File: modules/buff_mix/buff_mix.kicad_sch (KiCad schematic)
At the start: 2 parts

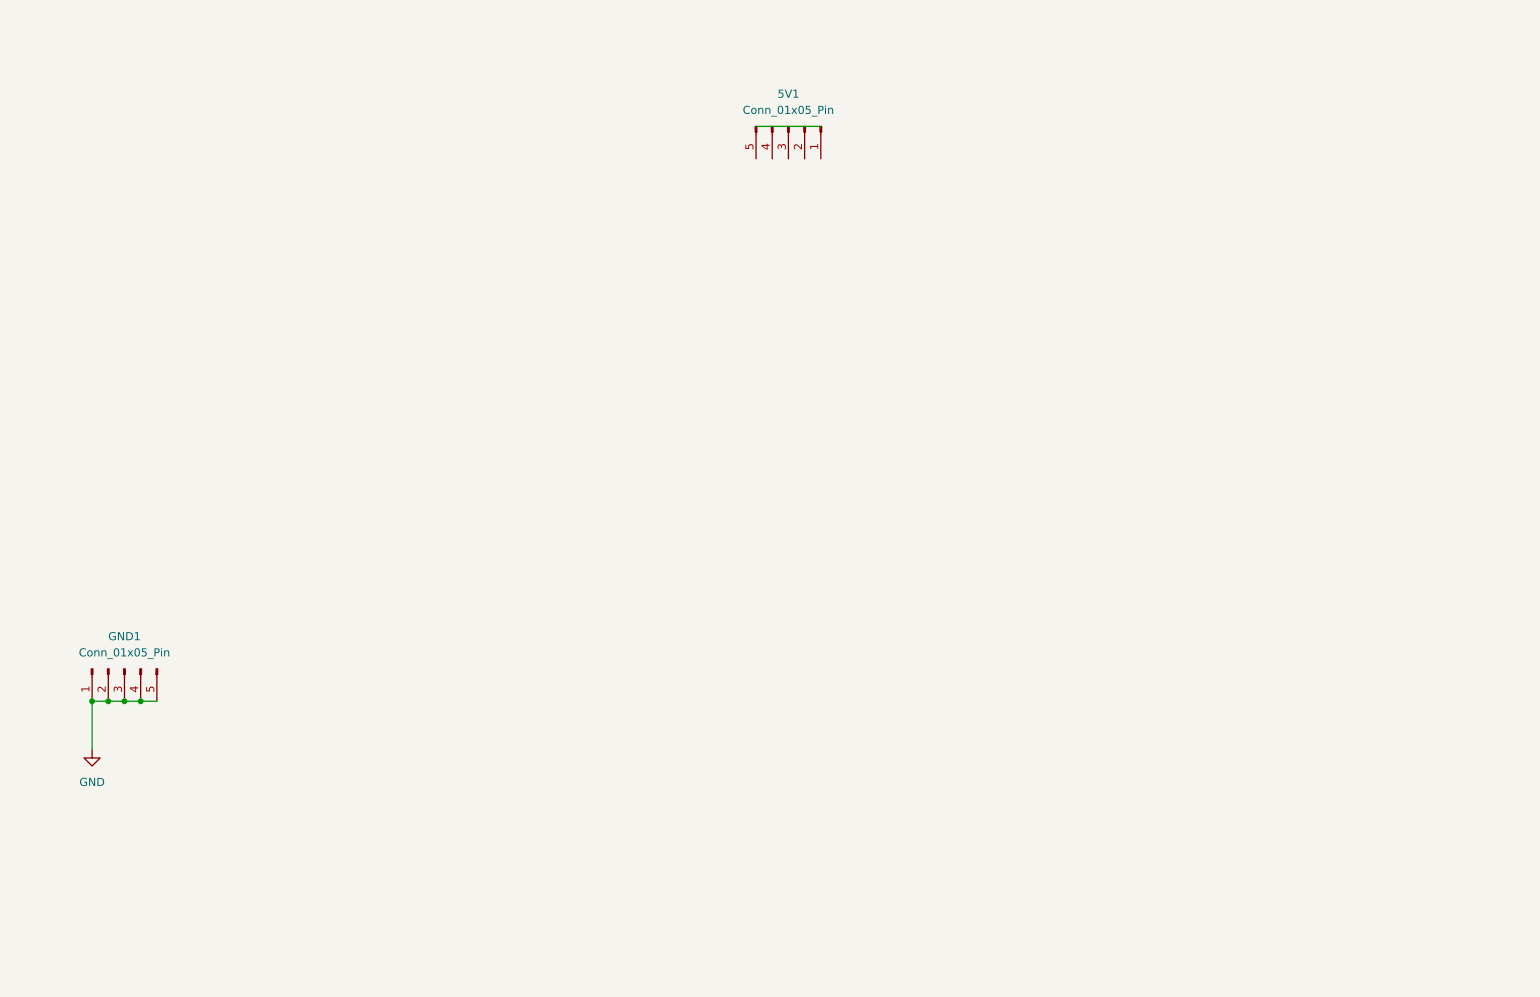
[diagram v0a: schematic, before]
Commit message: Add the final buff_mix
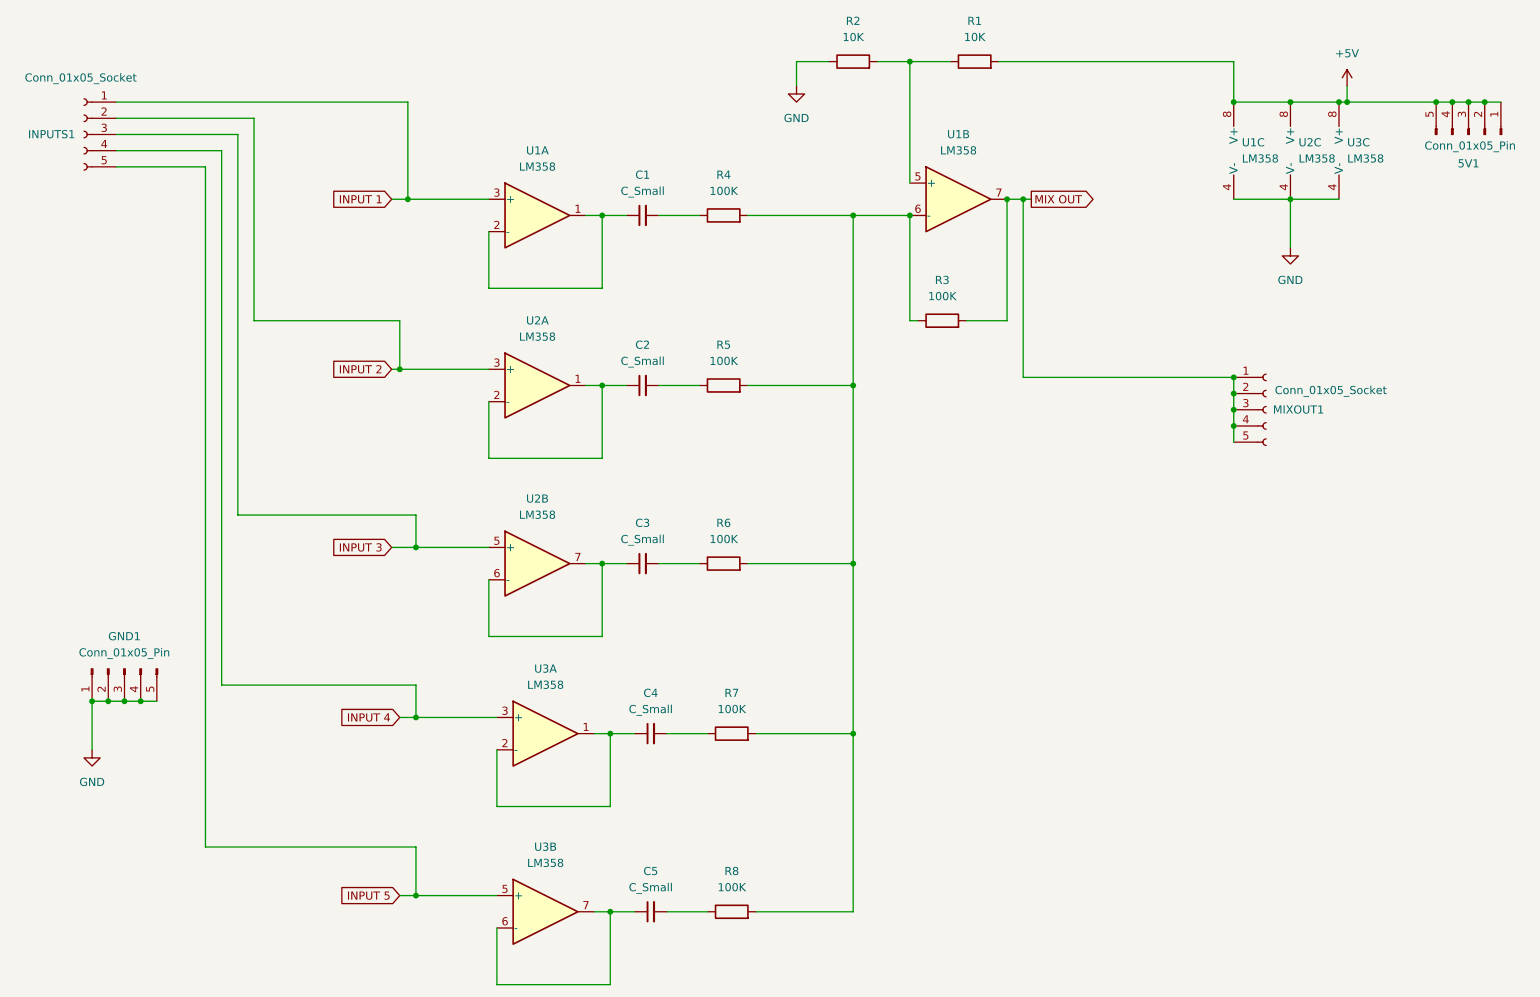
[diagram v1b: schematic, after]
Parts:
- added C1, C2, C3, C4, C5: C_Small, Capacitor_THT:C_Disc_D4.3mm_W1.9mm_P5.00mm, symbol Device:C_Small
- added INPUTS1, MIXOUT1: Conn_01x05_Socket, Connector_PinSocket_2.54mm:PinSocket_1x05_P2.54mm_Vertical, symbol Connector:Conn_01x05_Socket
- added R1, R2: 10K, Resistor_THT:R_Axial_DIN0207_L6.3mm_D2.5mm_P10.16mm_Horizontal, symbol Device:R
- added R3, R4, R5, R6, R7, R8: 100K, Resistor_THT:R_Axial_DIN0207_L6.3mm_D2.5mm_P10.16mm_Horizontal, symbol Device:R
- added U1, U2, U3: LM358, Library:LM358_THT, symbol Amplifier_Operational:LM358
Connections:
- net GND: now also R2.1, U1.4 (V-), U2.4 (V-), U3.4 (V-)
- net +5V: now reaches 5V1.1 (Pin_1)
- net +5V: now also 5V1.2 (Pin_2), 5V1.3 (Pin_3), 5V1.4 (Pin_4), 5V1.5 (Pin_5), R1.2, U1.8 (V+), U2.8 (V+), U3.8 (V+)
- new net: C3.2, R6.1
- new net: R3.1, R4.2, R5.2, R6.2, R7.2, R8.2, U1.6 (-)
- new net: C5.1, U3.6 (-), U3.7
- new net: C5.2, R8.1
- new net: C2.2, R5.1
- new net: C2.1, U2.1, U2.2 (-)
- new net: C1.2, R4.1
- new net: R1.1, R2.2, U1.5 (+)
- new net: C4.1, U3.1, U3.2 (-)
- new net: C4.2, R7.1
- new net: C3.1, U2.6 (-), U2.7
- new net: C1.1, U1.1, U1.2 (-)
- new net INPUT 1: INPUTS1.1 (Pin_1), U1.3 (+)
- new net INPUT 2: INPUTS1.2 (Pin_2), U2.3 (+)
- new net INPUT 3: INPUTS1.3 (Pin_3), U2.5 (+)
- new net INPUT 4: INPUTS1.4 (Pin_4), U3.3 (+)
- new net INPUT 5: INPUTS1.5 (Pin_5), U3.5 (+)
- new net MIX OUT: MIXOUT1.1 (Pin_1), MIXOUT1.2 (Pin_2), MIXOUT1.3 (Pin_3), MIXOUT1.4 (Pin_4), MIXOUT1.5 (Pin_5), R3.2, U1.7
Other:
- moved on the sheet: 5V1
